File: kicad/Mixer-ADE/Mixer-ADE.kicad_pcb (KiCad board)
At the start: 2 copper layers, 121 x 83 mm, 32 parts, among them J1 Audio_Jack, J2 BNC, J3 BNC, J6 BNC, M1 ADEX-10L, M2 ADEX-10L, T3 T37_XFRM

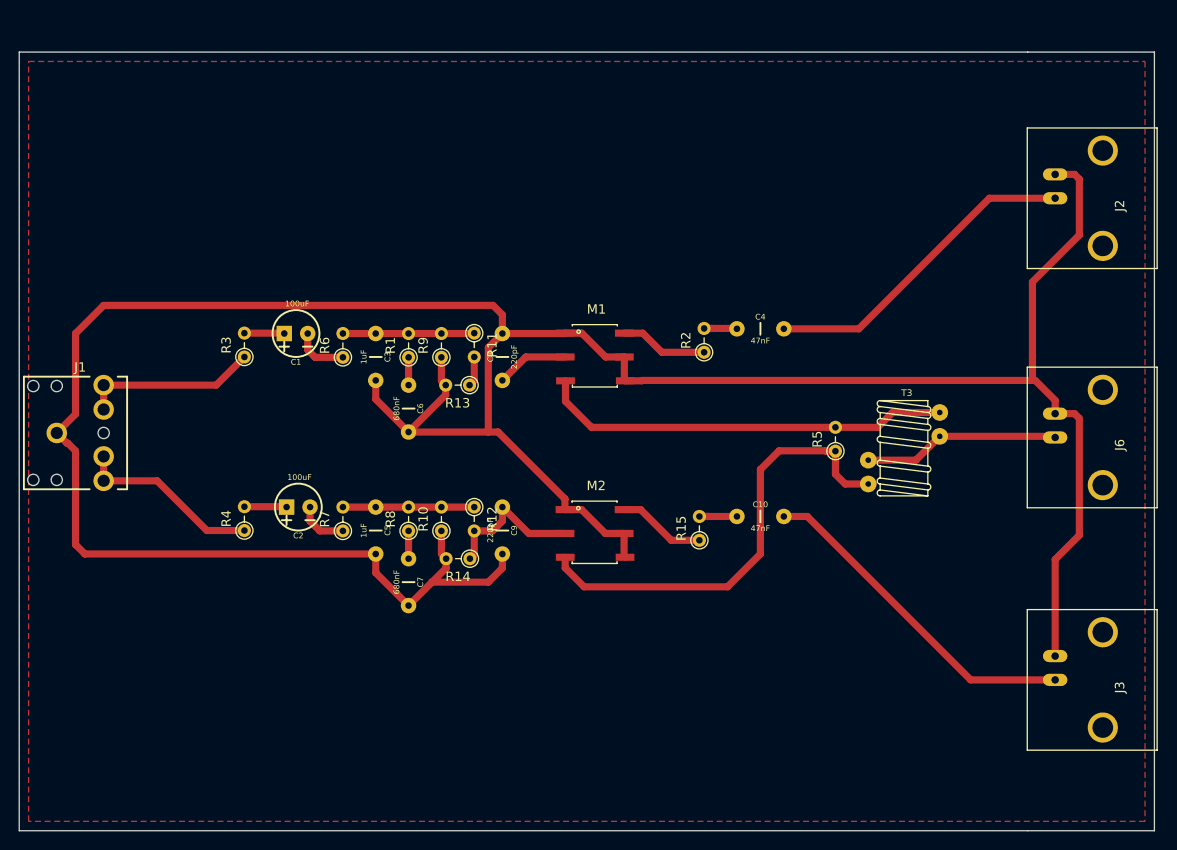
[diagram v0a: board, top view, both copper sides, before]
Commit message: Update Mixer-ADE.kicad_pcb
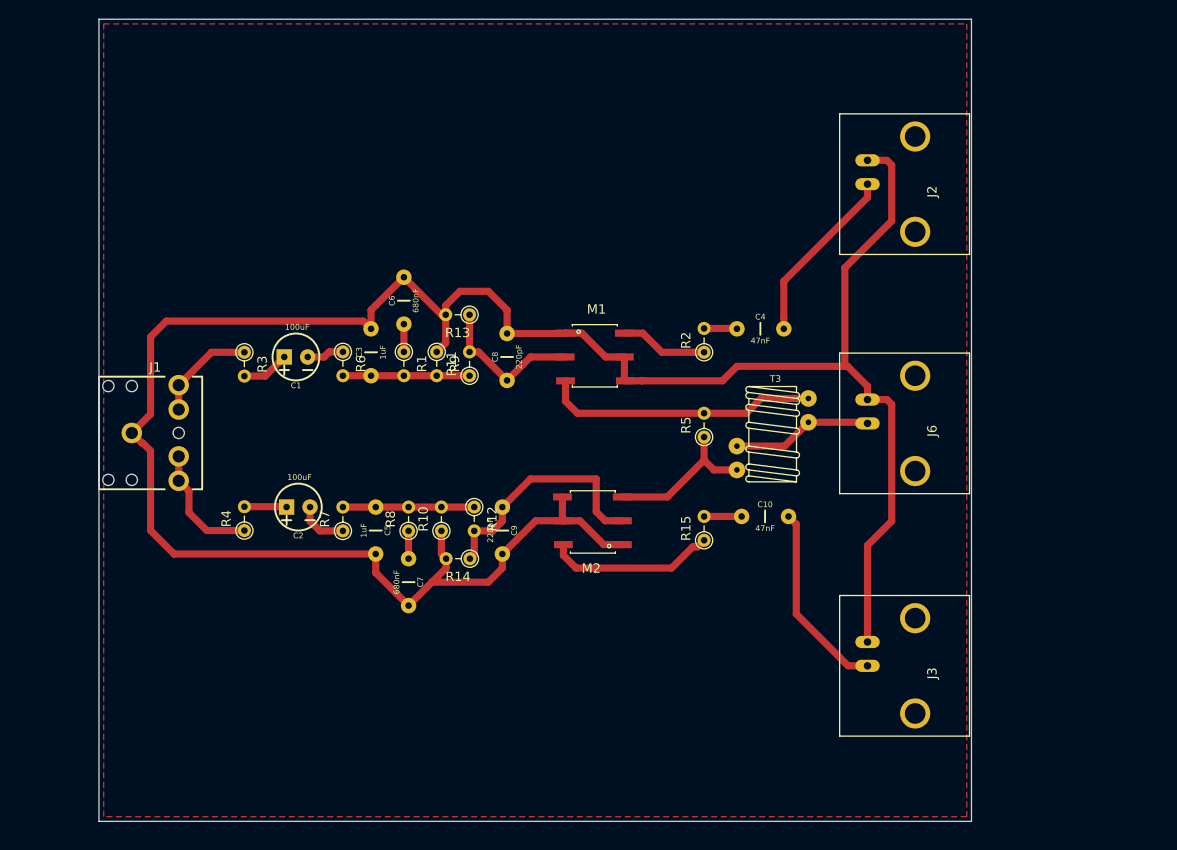
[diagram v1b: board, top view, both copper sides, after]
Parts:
- moved J2 20.1 mm to (172.8, 67.2)
- moved J3 20.1 mm to (172.8, 118.5)
- moved J6 20.1 mm to (172.8, 92.7)
- moved R5 14.1 mm to (151.5, 94.0)
- moved T3 14.1 mm to (158.8, 86.7)
- moved C6 11.5 mm to (119.5, 79.5), turned to 90 degrees
- moved J1 8.00 mm to (92.5, 85.1)
- moved R13 7.50 mm to (126.5, 81.0)
- moved M2 6.29 mm to (139.5, 106.8), turned to 180 degrees
- moved R11 4.57 mm to (126.5, 87.5), turned to 90 degrees
- moved C1 2.50 mm to (108.0, 85.5)
- moved R1 0.77 mm to (119.5, 85.0), turned to 270 degrees
- moved R9 0.77 mm to (123.0, 85.0), turned to 270 degrees
- moved C3 0.71 mm to (116.0, 85.0), turned to 90 degrees
- moved R6 0.58 mm to (113.0, 85.0), turned to 270 degrees
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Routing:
- net GND: track 311.0 -> 245.7 mm
- net Net-(M2-Pad3): track 48.5 -> 16.7 mm
- net Net-(C4-Pad2): track 34.7 -> 19.1 mm
- net Net-(C10-Pad2): track 36.1 -> 20.6 mm
- net Net-(M1-Pad3): track 43.9 -> 29.3 mm
- net Net-(C9-Pad1): track 15.9 -> 26.0 mm
- net Net-(M2-Pad6): track 9.38 -> 17.9 mm
- net Q_IN: track 18.8 -> 11.0 mm
- net I_IN: track 19.8 -> 13.1 mm
- net Net-(J6-PadS): track 21.0 -> 15.0 mm
- net Net-(C8-Pad1): track 10.9 -> 16.5 mm
- net Net-(C1-Pad2): track 5.83 -> 3.97 mm
- net Net-(C1-Pad1): track 4.27 -> 5.15 mm
- net Net-(C3-Pad1): track 14.0 -> 13.5 mm
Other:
- board size 121 x 83 mm -> 93 x 85.5 mm
